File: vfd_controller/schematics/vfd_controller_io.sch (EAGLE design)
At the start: 23 parts, among them IC1 HCPL-7840, IC2 HCPL-7840, IC3 MPC3201, IC4 MPC3201, IC5 MPC3201, IC6 MPC3201, X1 JST-XH-02-PIN-LONG-PAD, X2 JST-XH-02-PIN-LONG-PAD, X3 JST-XH-03-PIN-LONG-PAD, X4 JST-XH-03-PIN-LONG-PAD, X5 JST-XH-10-PIN-LONG-PAD, X6 JST-XH-02-PIN-LONG-PAD, X7 JST-XH-02-PIN-LONG-PAD

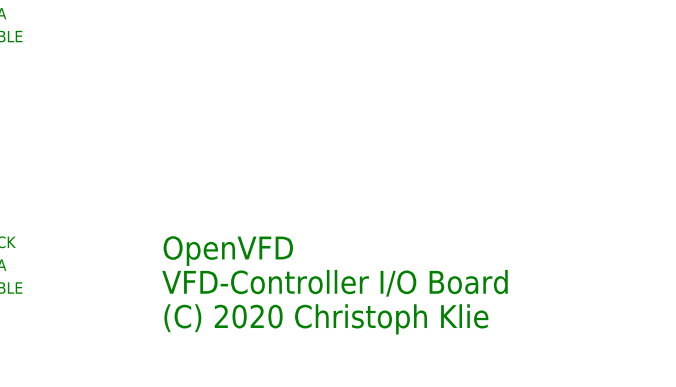
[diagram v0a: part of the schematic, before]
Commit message: Minor changes to Schematics Changed IGBT-Driver signal-side connector to plugs Updated Schematic Information Field
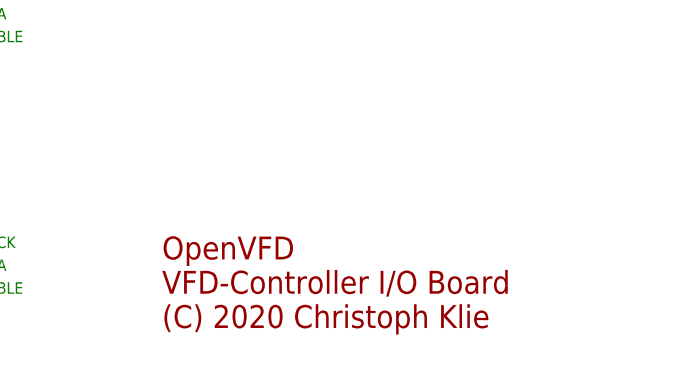
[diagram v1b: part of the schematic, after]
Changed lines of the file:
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@@
 <text x="7.62" y="73.66" size="1.27" layer="91" rot="R270">TEMPERATURE 1</text>
 <text x="7.62" y="45.72" size="1.27" layer="91" rot="R270">TEMPERATURE 2</text>
-<text x="163.83" y="31.75" size="2.54" layer="91">OpenVFD</text>
-<text x="163.83" y="27.94" size="2.54" layer="91">VFD-Controller I/O Board</text>
-<text x="163.83" y="24.13" size="2.54" layer="91">(C) 2020 Christoph Klie</text>
+<text x="163.83" y="31.75" size="2.54" layer="94">OpenVFD</text>
+<text x="163.83" y="27.94" size="2.54" layer="94">VFD-Controller I/O Board</text>
+<text x="163.83" y="24.13" size="2.54" layer="94">(C) 2020 Christoph Klie</text>
 </plain>
 <instances>
